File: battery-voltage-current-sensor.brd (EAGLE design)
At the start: 100 x 100 mm, 18 parts, among them IC1 ACS758LCB-050B-PFF-T, IC2 LM2596S-5.0_NOPB

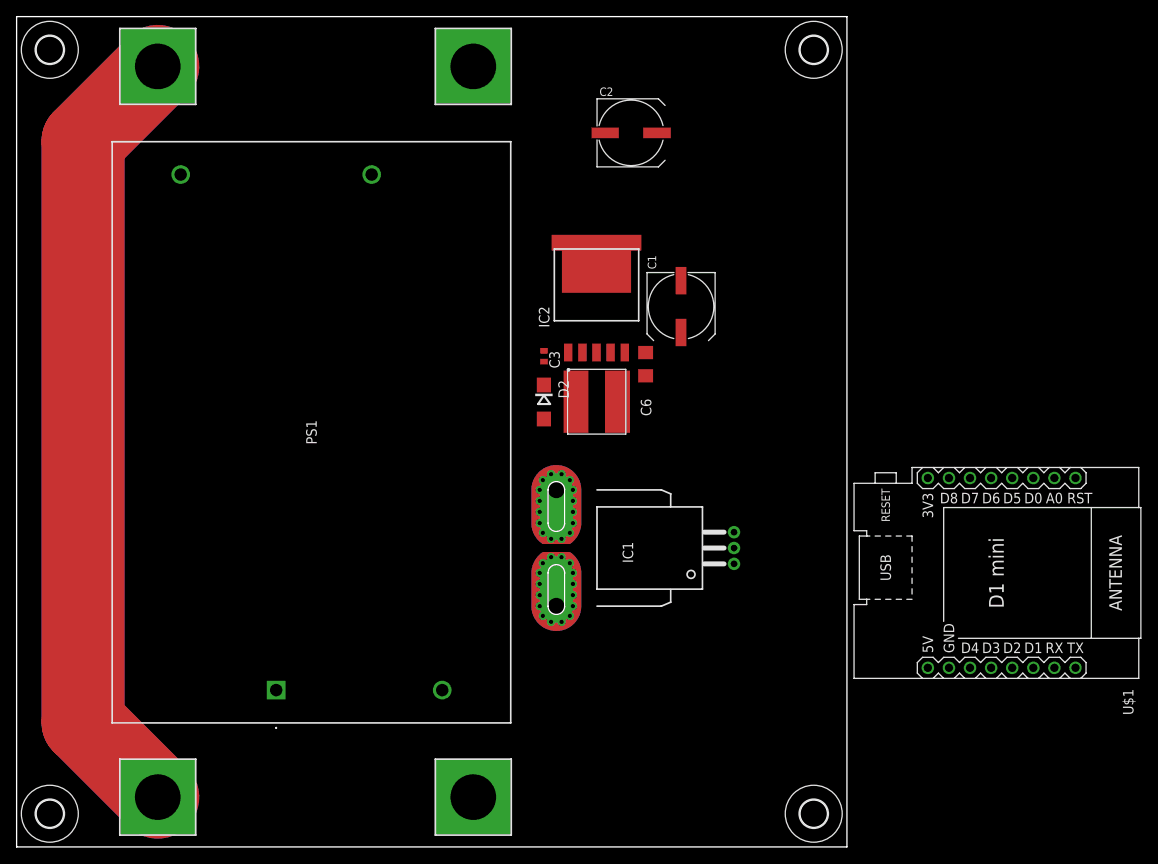
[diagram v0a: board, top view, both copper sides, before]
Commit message: first placing check
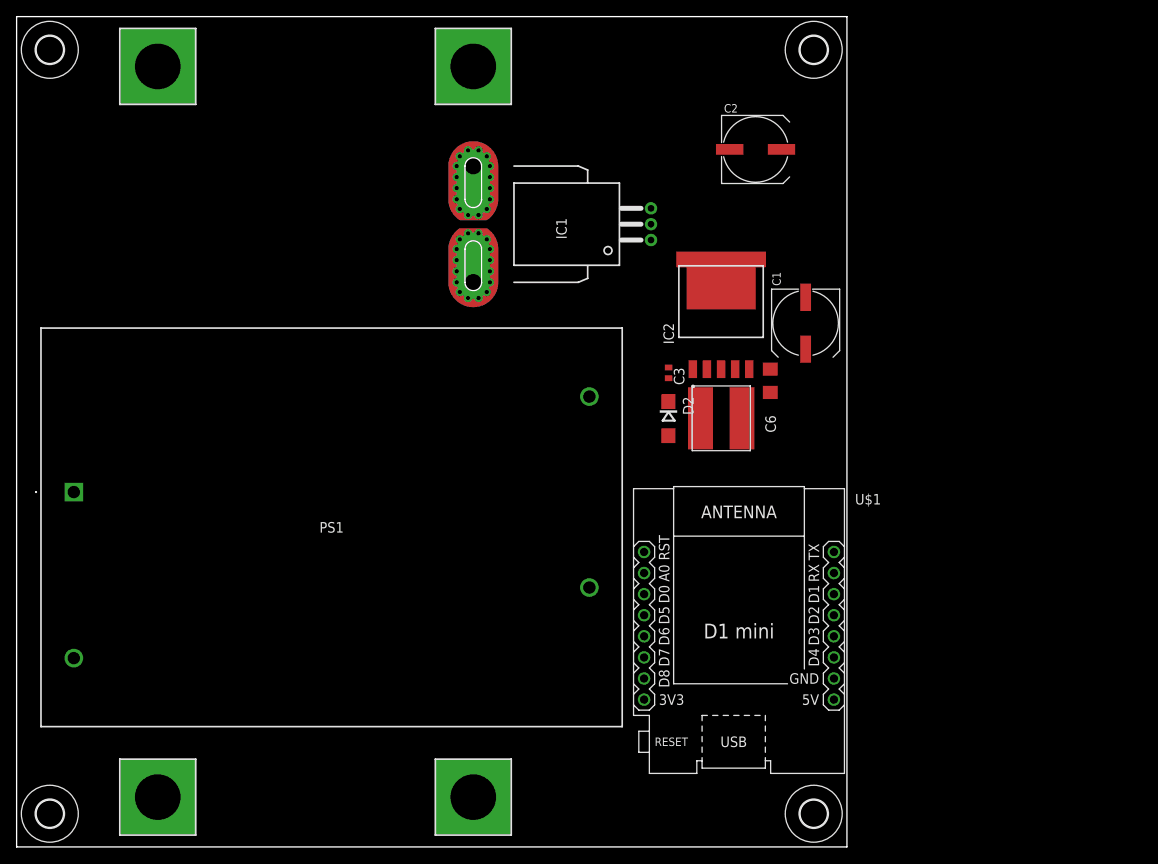
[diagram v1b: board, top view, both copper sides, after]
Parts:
- moved IC1 40.3 mm to (55.0, 75.0)
- moved PS1 34.1 mm to (6.89, 42.7), turned to 0 degrees
- moved U$1 31.8 mm to (87.0, 26.0), turned to 0 degrees
- moved C1 15.1 mm to (95.0, 63.1)
- moved C2 15.1 mm to (89.0, 84.0)
- moved C3 15.1 mm to (78.5, 57.1)
- moved C6 15.1 mm to (90.8, 56.1)
- moved D2 15.1 mm to (78.5, 51.6)
- moved IC2 15.1 mm to (84.8, 63.7)
- moved L2 15.1 mm to (84.9, 51.6)
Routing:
- net N$2: track 190.9 -> 0.00 mm
